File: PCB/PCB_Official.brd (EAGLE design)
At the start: 139.7 x 101.6 mm, 104 parts, among them IC1 MCP73871, J3 455-1750-1-ND, Q1 220mA/50V/3.5Ω, U1 TPS63070, U2 STM32F767ZIT6, U3 STM32L053C8T6, U4 TPS63070, U5 BATTERY-MANAGEMENT-TEMP_BQ274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

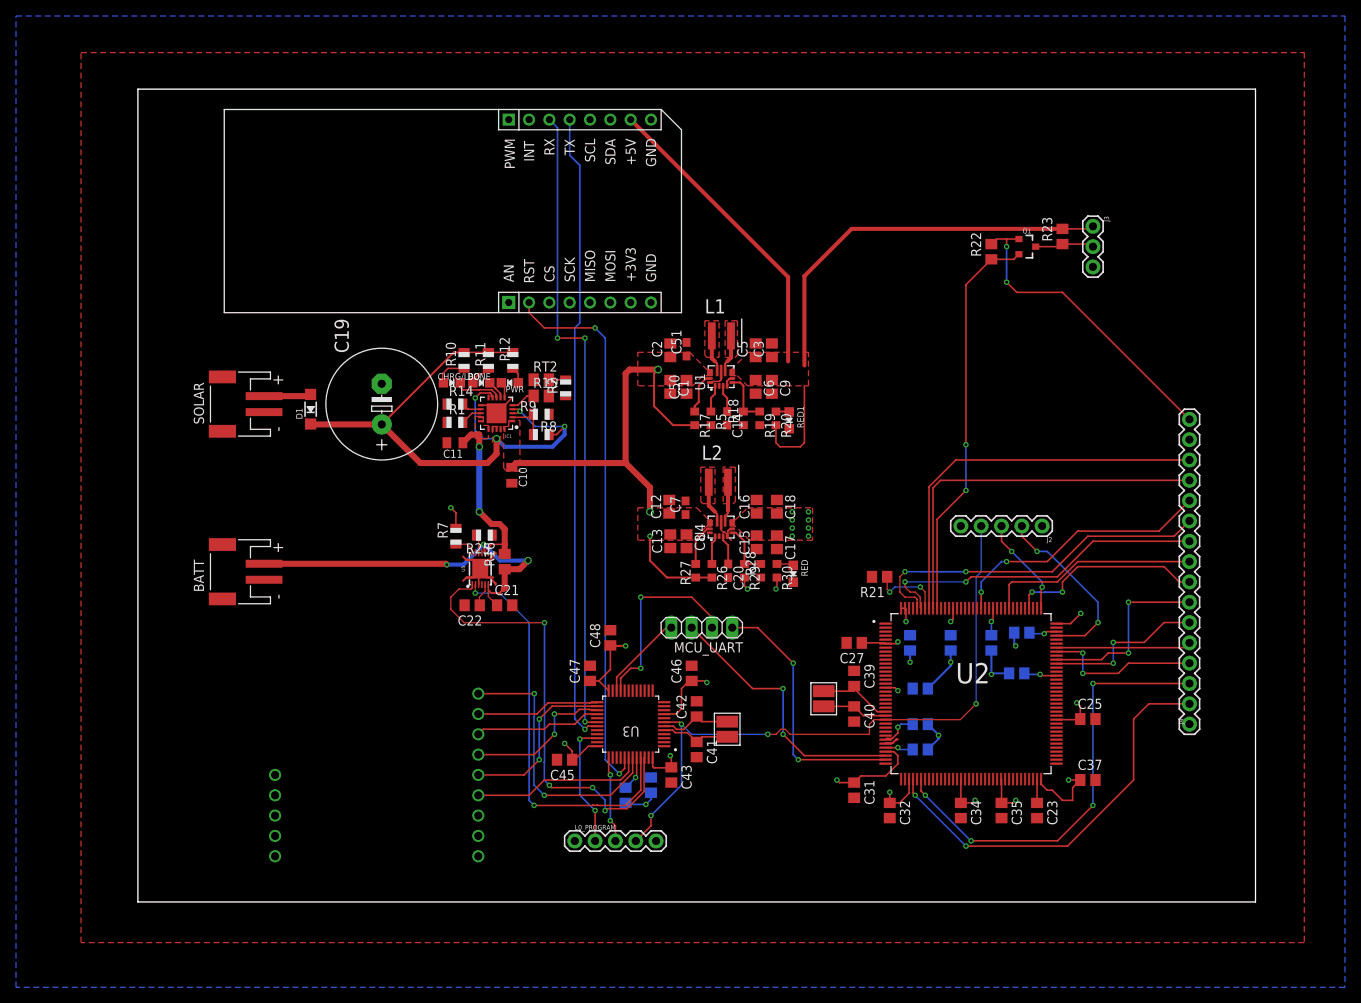
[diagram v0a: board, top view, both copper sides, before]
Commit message: Major revision after design review
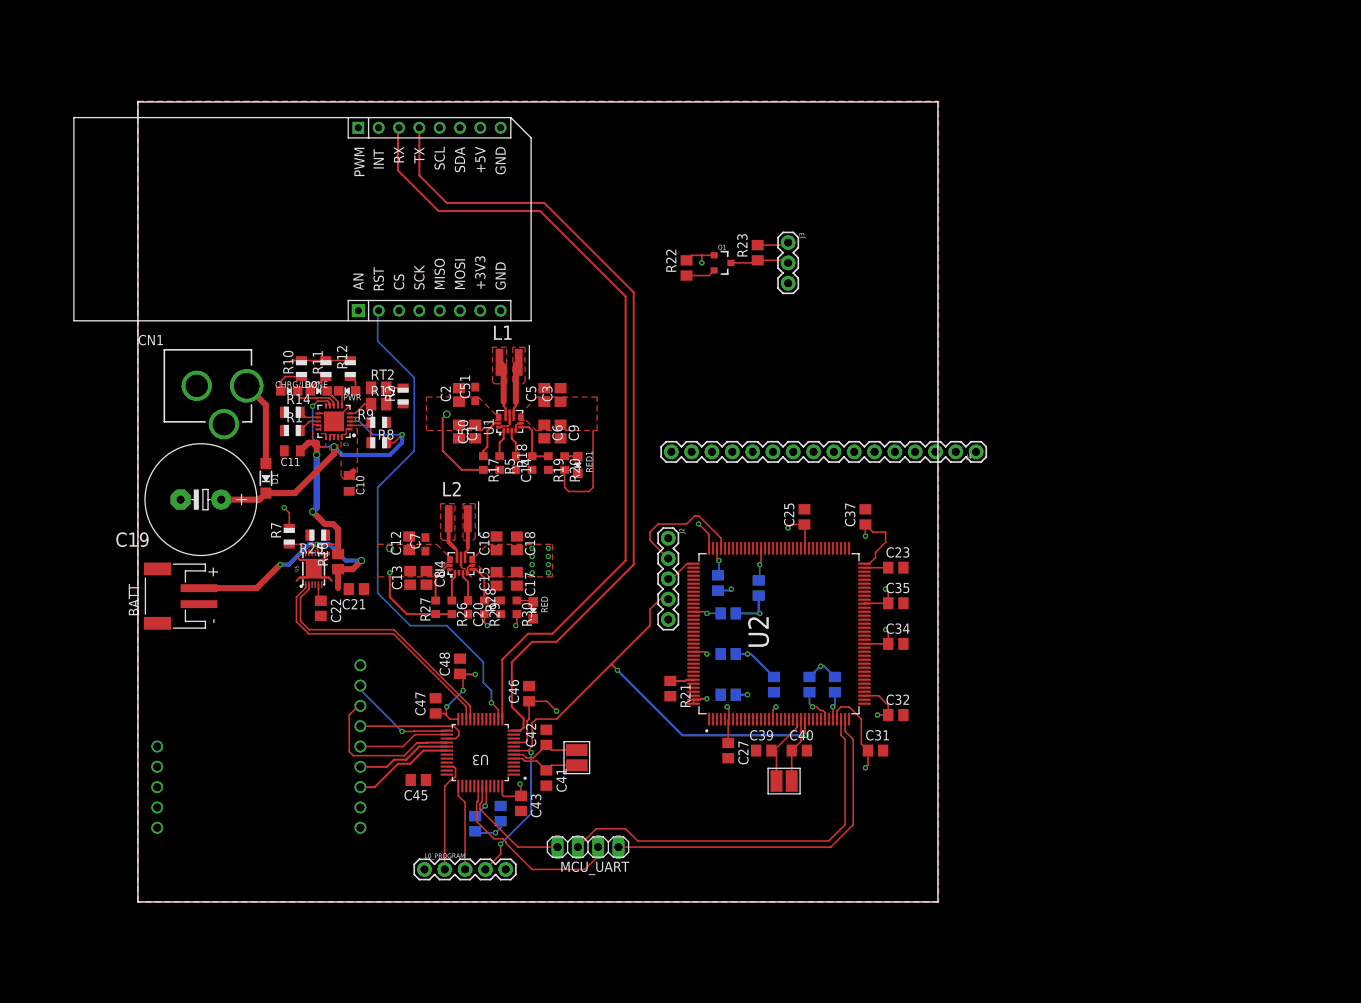
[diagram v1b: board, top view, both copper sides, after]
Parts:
- removed SOLAR: (no value), adafruit:JST-PH-2-SMT-RA
- added CN1: (no value), adafruit:DCJACK_2MM_PTH
- moved J2 46.8 mm to (66.3, 45.5), turned to 270 degrees
- moved C25 43.5 mm to (83.3, 48.1), turned to 90 degrees
- moved J4 43.2 mm to (104.8, 56.3), turned to 180 degrees
- moved C37 43.1 mm to (90.9, 48.1), turned to 90 degrees
- moved C24 38.5 mm to (72.5, 39.9), turned to 270 degrees
- moved R22 38.2 mm to (68.6, 79.2)
- moved J3 38.2 mm to (81.3, 82.4)
- moved Q1 38.2 mm to (73.0, 79.9)
- moved R23 38.2 mm to (77.5, 81.2)
- moved C23 35.1 mm to (94.7, 41.8), turned to 0 degrees
- moved C38 34.0 mm to (77.6, 39.2), turned to 270 degrees
- moved C28 33.1 mm to (73.8, 36.1), turned to 180 degrees
- moved C12 32.8 mm to (33.9, 44.8)
- moved C20 32.8 mm to (41.3, 36.8)
- moved L2 32.8 mm to (37.8, 46.1)
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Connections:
- new net LORA_EN: U$9.EN, U3.30
- net BAT_SCL: now also U3.21; no longer U3.45
- net BAT_SDA: now also U3.22; no longer U3.46
- net GND: now also CN1.GND, CN1.GNDBREAK; no longer SOLAR.2
- net GSM_RST: now also U3.14; no longer U3.41
- net L0_RX: now also U3.43; no longer U3.22
- net L0_TX: now also U3.42; no longer U3.21
- net LORA_INT: now also U3.29; no longer U3.42
- net LORA_RST: no longer U3.43
- net N$32: now also CN1.PWR; no longer SOLAR.1
- net RX_GSM: now also U3.13; no longer U3.30
- net TX_GSM: now also U3.12; no longer U3.31
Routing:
- net +5V: track 103.5 -> 19.3 mm
- net DCMI_PIXCLK: track 54.7 -> 0.00 mm, vias 4 -> 0
- net DCMI_HSYNC: track 50.9 -> 0.00 mm, vias 2 -> 0
- net I2C_SDA: track 49.1 -> 0.00 mm
- net I2C_SCL: track 47.5 -> 0.00 mm
- net TIM3_CH2: track 50.1 -> 3.71 mm, vias 2 -> 0
- net DCMI_D7: track 44.6 -> 0.00 mm, vias 2 -> 0
- net DCMI_D6: track 42.2 -> 0.00 mm, vias 2 -> 0
- net +3V3: track 148.0 -> 110.1 mm
- net VOUT_CHARGER: track 61.8 -> 25.3 mm
- net LORA_RST: track 34.4 -> 0.00 mm, vias 2 -> 0
- net DCMI_VSYNC: track 33.5 -> 0.03 mm, vias 2 -> 0
- net DCMI_D5: track 26.7 -> 0.00 mm
- net BAT_SDA: track 57.3 -> 32.3 mm, vias 4 -> 0
- net DCMI_D4: track 24.7 -> 0.00 mm, vias 2 -> 0
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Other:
- board size 139.7 x 101.6 mm -> 100 x 100 mm
